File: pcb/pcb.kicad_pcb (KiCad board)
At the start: 2 copper layers, 57 x 84 mm, 4 parts, among them J1 Botones, J2 Pedales+Velocimetro+Monedas, J3 Volante

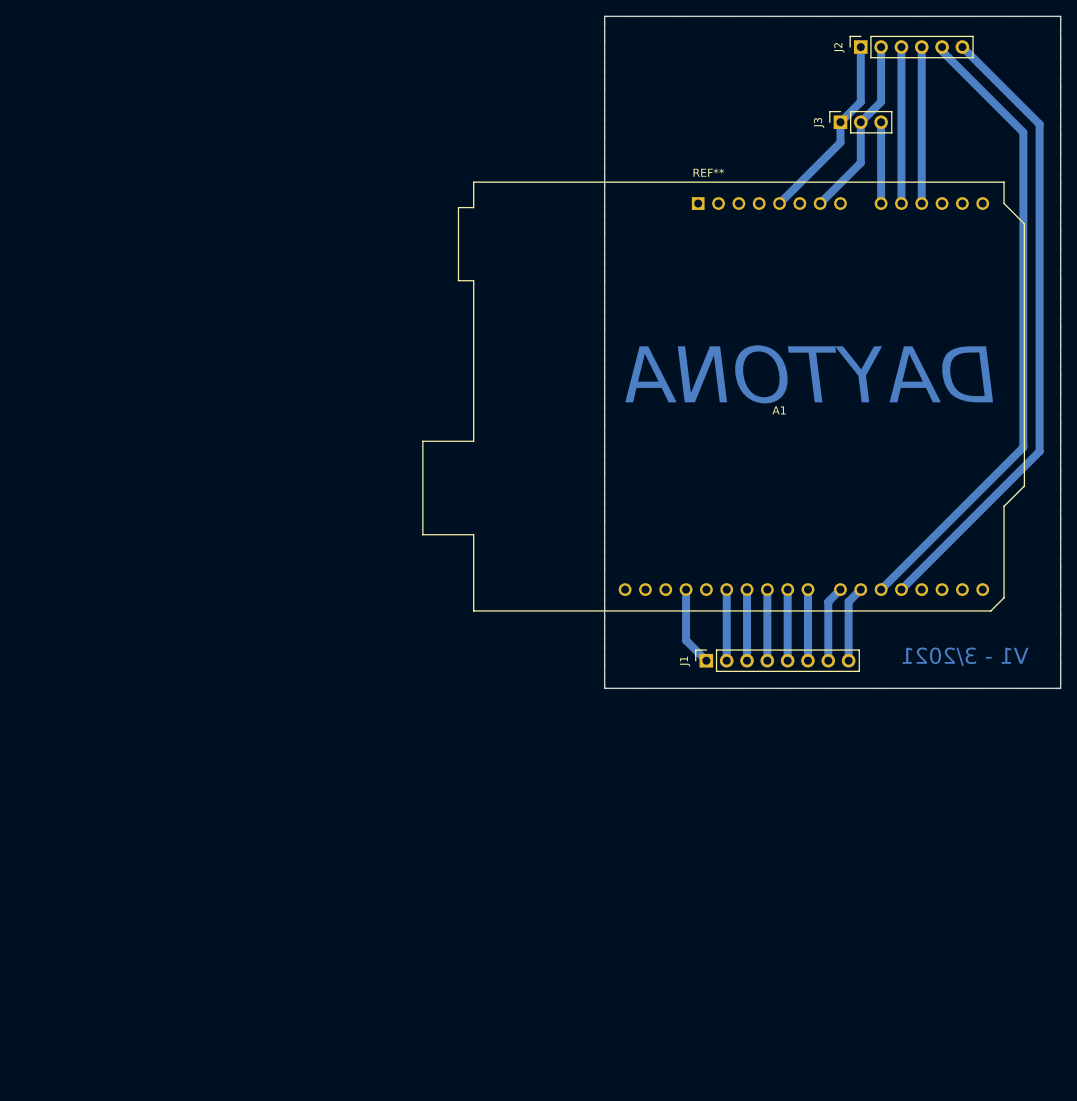
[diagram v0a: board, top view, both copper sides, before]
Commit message: Add layout and schematic prints
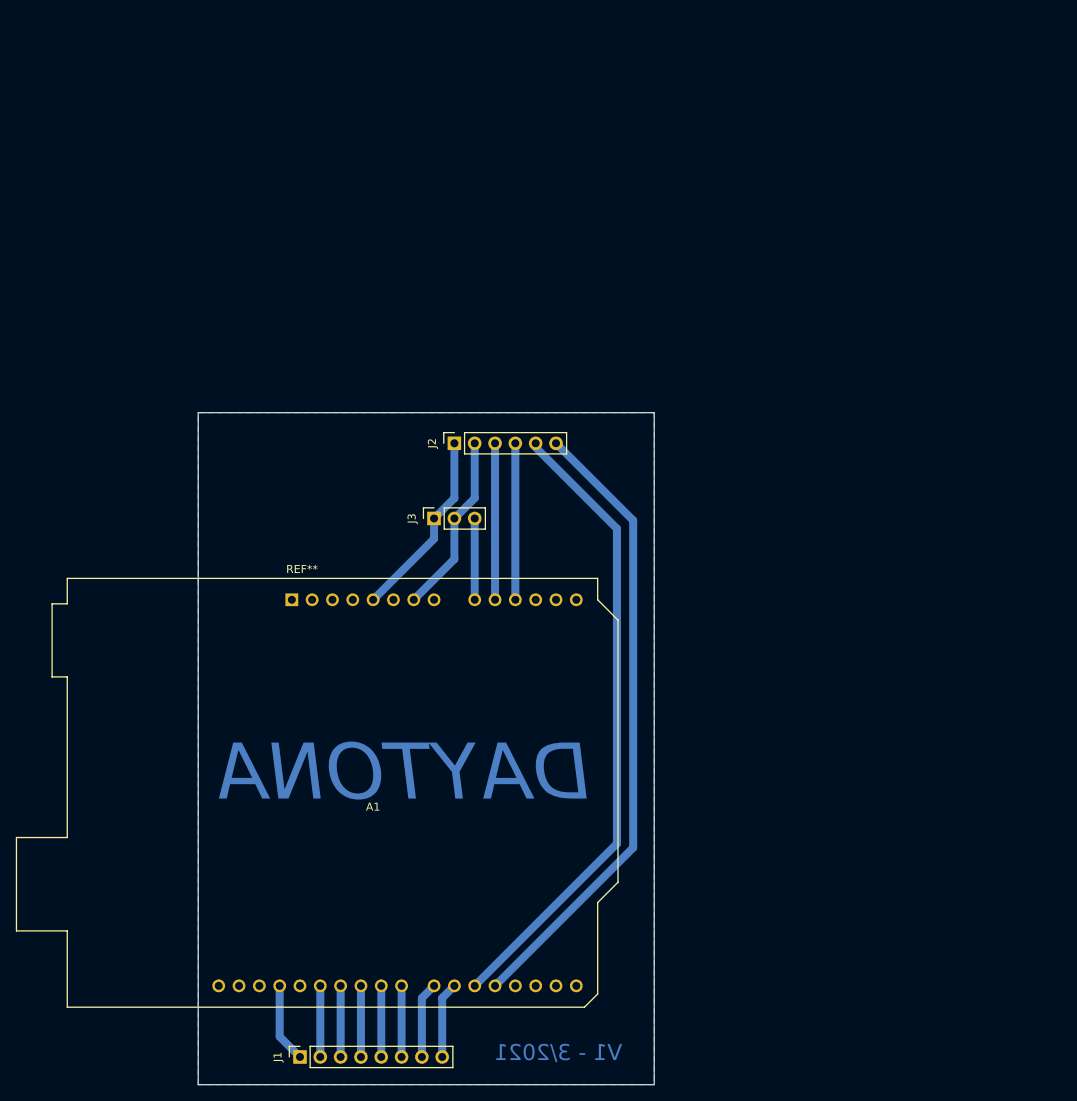
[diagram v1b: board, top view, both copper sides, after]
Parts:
- moved A1 70.9 mm to (99.1, 147.3)
- moved J1 70.9 mm to (89.9, 179.1)
- moved J2 70.9 mm to (109.2, 102.4)
- moved J3 70.9 mm to (106.7, 111.8)
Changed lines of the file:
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@@
     (thickness 1.6)
   )
-  (paper "A4")
+  (paper "A4" portrait)
+  (title_block
+    (title "Ches Pur Ofi")
+    (date "3/2021")
+    (rev "V1")
+  )
   (layers
     (0 "F.Cu" signal)
@@
   (net 32 "Net-(A1-Pad32)")
   (footprint "Connector_PinSocket_2.54mm:PinSocket_1x03_P2.54mm_Vertical" (layer "F.Cu")
-    (at 157.48 62.23 90)
+    (at 106.68 111.76 90)
     (descr "Through hole straight socket strip, 1x03, 2.54mm pitch, single row (from Kicad 4.0.7), script generated")
     (tags "Through hole socket strip THT 1x03 2.54mm single row")
@@
   )
   (footprint "luqas11:Arduino_Leonardo_WithFemaleSockets" (layer "F.Cu")
-    (at 149.86 97.79)
+    (at 99.06 147.32)
     (attr through_hole)
     (fp_text reference "A1" (at 0 0.5) (layer "F.SilkS")
@@
   )
   (footprint "Connector_PinSocket_2.54mm:PinSocket_1x08_P2.54mm_Vertical" (layer "F.Cu")
-    (at 140.716 129.54 90)
+    (at 89.916 179.07 90)
     (descr "Through hole straight socket strip, 1x08, 2.54mm pitch, single row (from Kicad 4.0.7), script generated")
     (tags "Through hole socket strip THT 1x08 2.54mm single row")
@@
   )
   (footprint "Connector_PinSocket_2.54mm:PinSocket_1x06_P2.54mm_Vertical" (layer "F.Cu")
-    (at 160.02 52.832 90)
+    (at 109.22 102.362 90)
     (descr "Through hole straight socket strip, 1x06, 2.54mm pitch, single row (from Kicad 4.0.7), script generated")
     (tags "Through hole socket strip THT 1x06 2.54mm single row")
@@
     )
   )
-  (gr_line (start 128 49) (end 185 49)
+  (gr_line (start 77.2 98.53) (end 134.2 98.53)
     (stroke (width 0.1) (type solid)) (layer "Edge.Cuts"))
-  (gr_line (start 185 49) (end 185 133)
+  (gr_line (start 134.2 98.53) (end 134.2 182.53)
     (stroke (width 0.1) (type solid)) (layer "Edge.Cuts"))
-  (gr_line (start 185 133) (end 128 133)
+  (gr_line (start 134.2 182.53) (end 77.2 182.53)
     (stroke (width 0.1) (type solid)) (layer "Edge.Cuts"))
-  (gr_line (start 128 133) (end 128 49)
+  (gr_line (start 77.2 182.53) (end 77.2 98.53)
     (stroke (width 0.1) (type solid)) (layer "Edge.Cuts"))
-  (gr_text "V1 - 3/2021" (at 173 129) (layer "B.Cu")
+  (gr_text "V1 - 3/2021" (at 122.2 178.53) (layer "B.Cu")
     (effects (font (size 2 2) (thickness 0.5)) (justify mirror))
   )
-  (gr_text "DAYTONA" (at 154 94) (layer "B.Cu")
+  (gr_text "DAYTONA" (at 103.2 143.53) (layer "B.Cu")
     (effects (font (size 7 7) (thickness 1.3) italic) (justify mirror))
   )
-  (segment (start 138.18 127.004) (end 140.716 129.54) (width 1) (layer "B.Cu") (net 5))
-  (segment (start 138.18 120.65) (end 138.18 127.004) (width 1) (layer "B.Cu") (net 5))
-  (segment (start 143.26 129.536) (end 143.256 129.54) (width 1) (layer "B.Cu") (net 9))
-  (segment (start 143.26 120.65) (end 143.26 129.536) (width 1) (layer "B.Cu") (net 9))
-  (segment (start 167.64 53.34) (end 167.64 72.39) (width 1) (layer "B.Cu") (net 10))
-  (segment (start 145.8 120.65) (end 145.8 129.536) (width 1) (layer "B.Cu") (net 11))
-  (segment (start 145.8 129.536) (end 145.796 129.54) (width 1) (layer "B.Cu") (net 11))
-  (segment (start 165.1 53.34) (end 165.1 72.39) (width 1) (layer "B.Cu") (net 12))
-  (segment (start 148.34 120.65) (end 148.34 129.536) (width 1) (layer "B.Cu") (net 13))
-  (segment (start 148.34 129.536) (end 148.336 129.54) (width 1) (layer "B.Cu") (net 13))
-  (segment (start 162.56 62.23) (end 162.56 72.39) (width 1) (layer "B.Cu") (net 14))
-  (segment (start 150.88 129.536) (end 150.876 129.54) (width 1) (layer "B.Cu") (net 15))
-  (segment (start 150.88 120.65) (end 150.88 129.536) (width 1) (layer "B.Cu") (net 15))
-  (segment (start 153.42 120.65) (end 153.42 129.536) (width 1) (layer "B.Cu") (net 17))
-  (segment (start 153.42 129.536) (end 153.416 129.54) (width 1) (layer "B.Cu") (net 17))
-  (segment (start 160.02 62.23) (end 160.02 67.31) (width 1) (layer "B.Cu") (net 18))
-  (segment (start 162.56 59.69) (end 160.02 62.23) (width 1) (layer "B.Cu") (net 18))
-  (segment (start 162.56 53.34) (end 162.56 59.69) (width 1) (layer "B.Cu") (net 18))
-  (segment (start 160.02 67.31) (end 154.94 72.39) (width 1) (layer "B.Cu") (net 18))
-  (segment (start 155.956 122.174) (end 155.956 129.54) (width 1) (layer "B.Cu") (net 19))
-  (segment (start 157.48 120.65) (end 155.956 122.174) (width 1) (layer "B.Cu") (net 19))
-  (segment (start 160.02 120.65) (end 158.496 122.174) (width 1) (layer "B.Cu") (net 21))
-  (segment (start 158.496 122.174) (end 158.496 129.54) (width 1) (layer "B.Cu") (net 21))
-  (segment (start 160.02 53.34) (end 160.02 59.69) (width 1) (layer "B.Cu") (net 22))
-  (segment (start 157.48 62.23) (end 157.48 64.77) (width 1) (layer "B.Cu") (net 22))
-  (segment (start 150.179998 72.39) (end 149.86 72.39) (width 1) (layer "B.Cu") (net 22))
-  (segment (start 160.02 59.69) (end 157.48 62.23) (width 1) (layer "B.Cu") (net 22))
-  (segment (start 157.48 64.77) (end 149.86 72.39) (width 1) (layer "B.Cu") (net 22))
-  (segment (start 170.18 53.34) (end 180.34 63.5) (width 1) (layer "B.Cu") (net 23))
-  (segment (start 180.34 63.5) (end 180.34 102.87) (width 1) (layer "B.Cu") (net 23))
-  (segment (start 180.34 102.87) (end 162.56 120.65) (width 1) (layer "B.Cu") (net 23))
-  (segment (start 182.372 103.378) (end 165.1 120.65) (width 1) (layer "B.Cu") (net 25))
-  (segment (start 182.372 62.484) (end 182.372 103.378) (width 1) (layer "B.Cu") (net 25))
-  (segment (start 172.72 52.832) (end 182.372 62.484) (width 1) (layer "B.Cu") (net 25))
+  (segment (start 87.38 176.534) (end 89.916 179.07) (width 1) (layer "B.Cu") (net 5))
+  (segment (start 87.38 170.18) (end 87.38 176.534) (width 1) (layer "B.Cu") (net 5))
+  (segment (start 92.46 179.066) (end 92.456 179.07) (width 1) (layer "B.Cu") (net 9))
+  (segment (start 92.46 170.18) (end 92.46 179.066) (width 1) (layer "B.Cu") (net 9))
+  (segment (start 116.84 102.87) (end 116.84 121.92) (width 1) (layer "B.Cu") (net 10))
+  (segment (start 95 170.18) (end 95 179.066) (width 1) (layer "B.Cu") (net 11))
+  (segment (start 95 179.066) (end 94.996 179.07) (width 1) (layer "B.Cu") (net 11))
+  (segment (start 114.3 102.87) (end 114.3 121.92) (width 1) (layer "B.Cu") (net 12))
+  (segment (start 97.54 170.18) (end 97.54 179.066) (width 1) (layer "B.Cu") (net 13))
+  (segment (start 97.54 179.066) (end 97.536 179.07) (width 1) (layer "B.Cu") (net 13))
+  (segment (start 111.76 111.76) (end 111.76 121.92) (width 1) (layer "B.Cu") (net 14))
+  (segment (start 100.08 179.066) (end 100.076 179.07) (width 1) (layer "B.Cu") (net 15))
+  (segment (start 100.08 170.18) (end 100.08 179.066) (width 1) (layer "B.Cu") (net 15))
+  (segment (start 102.62 170.18) (end 102.62 179.066) (width 1) (layer "B.Cu") (net 17))
+  (segment (start 102.62 179.066) (end 102.616 179.07) (width 1) (layer "B.Cu") (net 17))
+  (segment (start 109.22 111.76) (end 109.22 116.84) (width 1) (layer "B.Cu") (net 18))
+  (segment (start 111.76 109.22) (end 109.22 111.76) (width 1) (layer "B.Cu") (net 18))
+  (segment (start 111.76 102.87) (end 111.76 109.22) (width 1) (layer "B.Cu") (net 18))
+  (segment (start 109.22 116.84) (end 104.14 121.92) (width 1) (layer "B.Cu") (net 18))
+  (segment (start 105.156 171.704) (end 105.156 179.07) (width 1) (layer "B.Cu") (net 19))
+  (segment (start 106.68 170.18) (end 105.156 171.704) (width 1) (layer "B.Cu") (net 19))
+  (segment (start 109.22 170.18) (end 107.696 171.704) (width 1) (layer "B.Cu") (net 21))
+  (segment (start 107.696 171.704) (end 107.696 179.07) (width 1) (layer "B.Cu") (net 21))
+  (segment (start 109.22 102.87) (end 109.22 109.22) (width 1) (layer "B.Cu") (net 22))
+  (segment (start 106.68 111.76) (end 106.68 114.3) (width 1) (layer "B.Cu") (net 22))
+  (segment (start 99.379998 121.92) (end 99.06 121.92) (width 1) (layer "B.Cu") (net 22))
+  (segment (start 109.22 109.22) (end 106.68 111.76) (width 1) (layer "B.Cu") (net 22))
+  (segment (start 106.68 114.3) (end 99.06 121.92) (width 1) (layer "B.Cu") (net 22))
+  (segment (start 119.38 102.87) (end 129.54 113.03) (width 1) (layer "B.Cu") (net 23))
+  (segment (start 129.54 113.03) (end 129.54 152.4) (width 1) (layer "B.Cu") (net 23))
+  (segment (start 129.54 152.4) (end 111.76 170.18) (width 1) (layer "B.Cu") (net 23))
+  (segment (start 131.572 152.908) (end 114.3 170.18) (width 1) (layer "B.Cu") (net 25))
+  (segment (start 131.572 112.014) (end 131.572 152.908) (width 1) (layer "B.Cu") (net 25))
+  (segment (start 121.92 102.362) (end 131.572 112.014) (width 1) (layer "B.Cu") (net 25))
   (zone (net 0) (net_name "") (layer "B.Cu") (hatch edge 0.508)
     (connect_pads (clearance 2))
@@
     (polygon
       (pts
-        (xy 185 133)
-        (xy 128 133)
-        (xy 128 49)
-        (xy 185 49)
+        (xy 134.2 182.53)
+        (xy 77.2 182.53)
+        (xy 77.2 98.53)
+        (xy 134.2 98.53)
       )
     )
